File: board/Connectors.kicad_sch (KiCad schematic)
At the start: 17 parts, among them J10 SLOT 1, J11 SLOT 2, J12 SLOT 3, J13 SLOT 4, J14 SLOT 5, J15 Audio Jack, J16 SPI Device 0, J18 SPI Device 1, J19 SPI Device 2, J20 SPI Device 3, J21 SPI Device 4, J22 SPI Device 5, J23 SPI Device 6, J24 SPI Device 7, J25 VIA Port A, J26 SP720APP, J9 SLOT 0

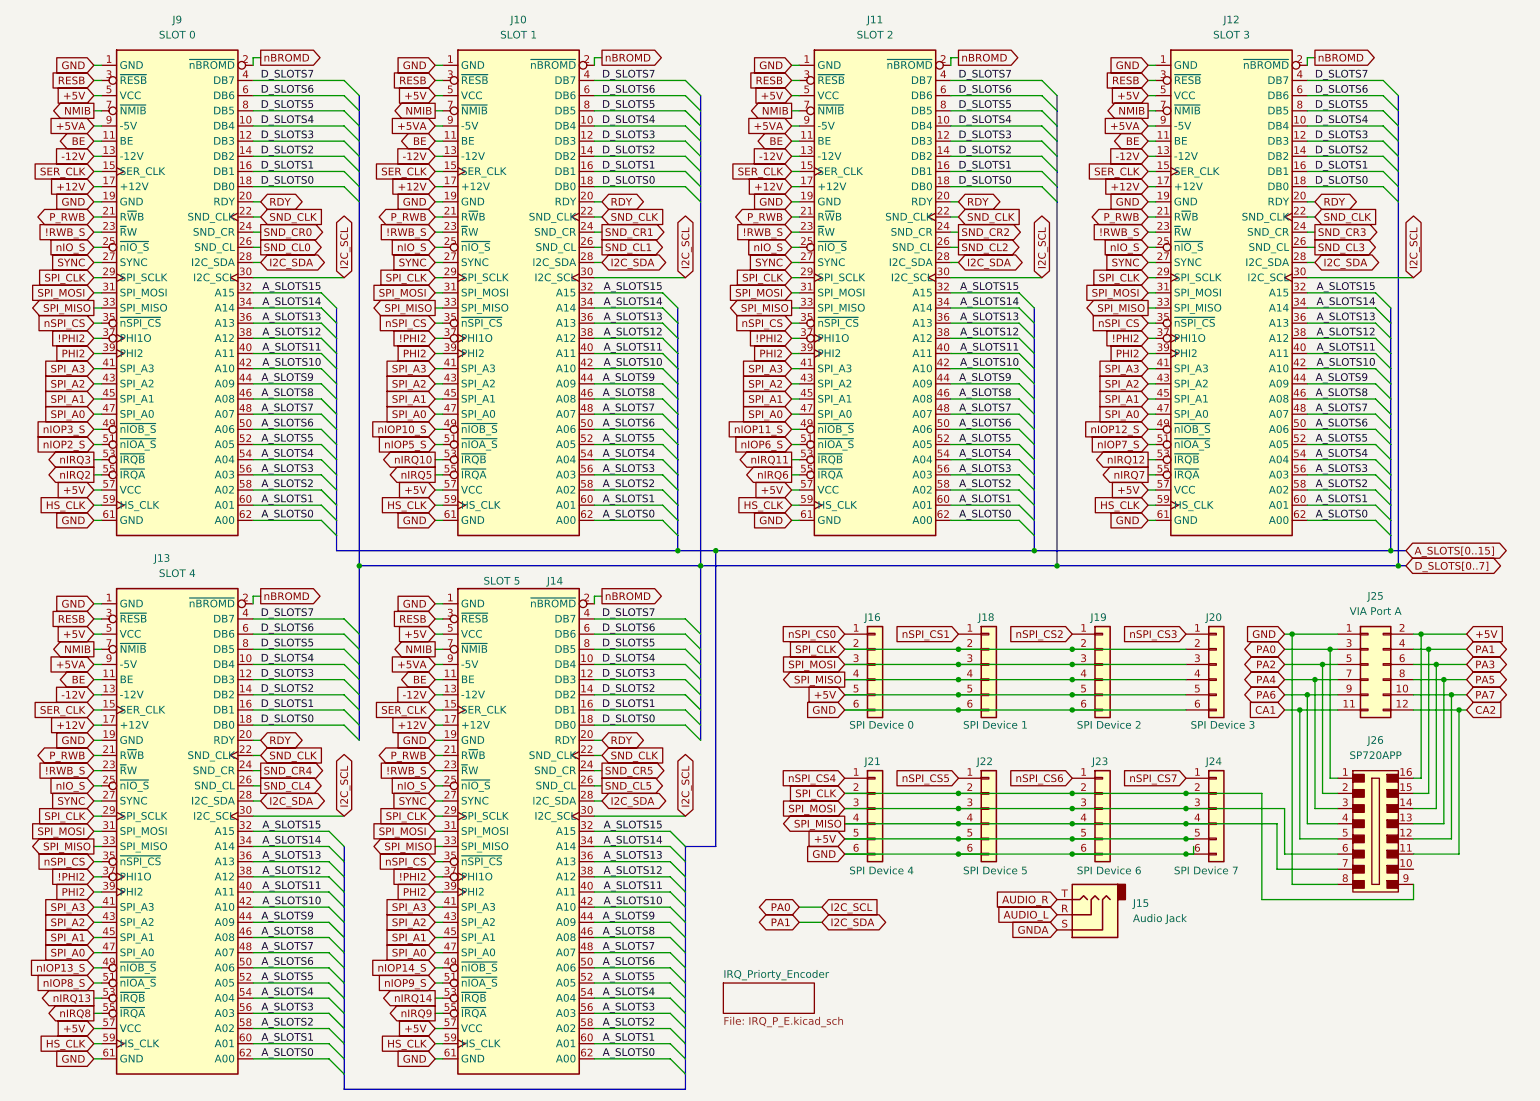
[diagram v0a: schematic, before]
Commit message: V1.4E
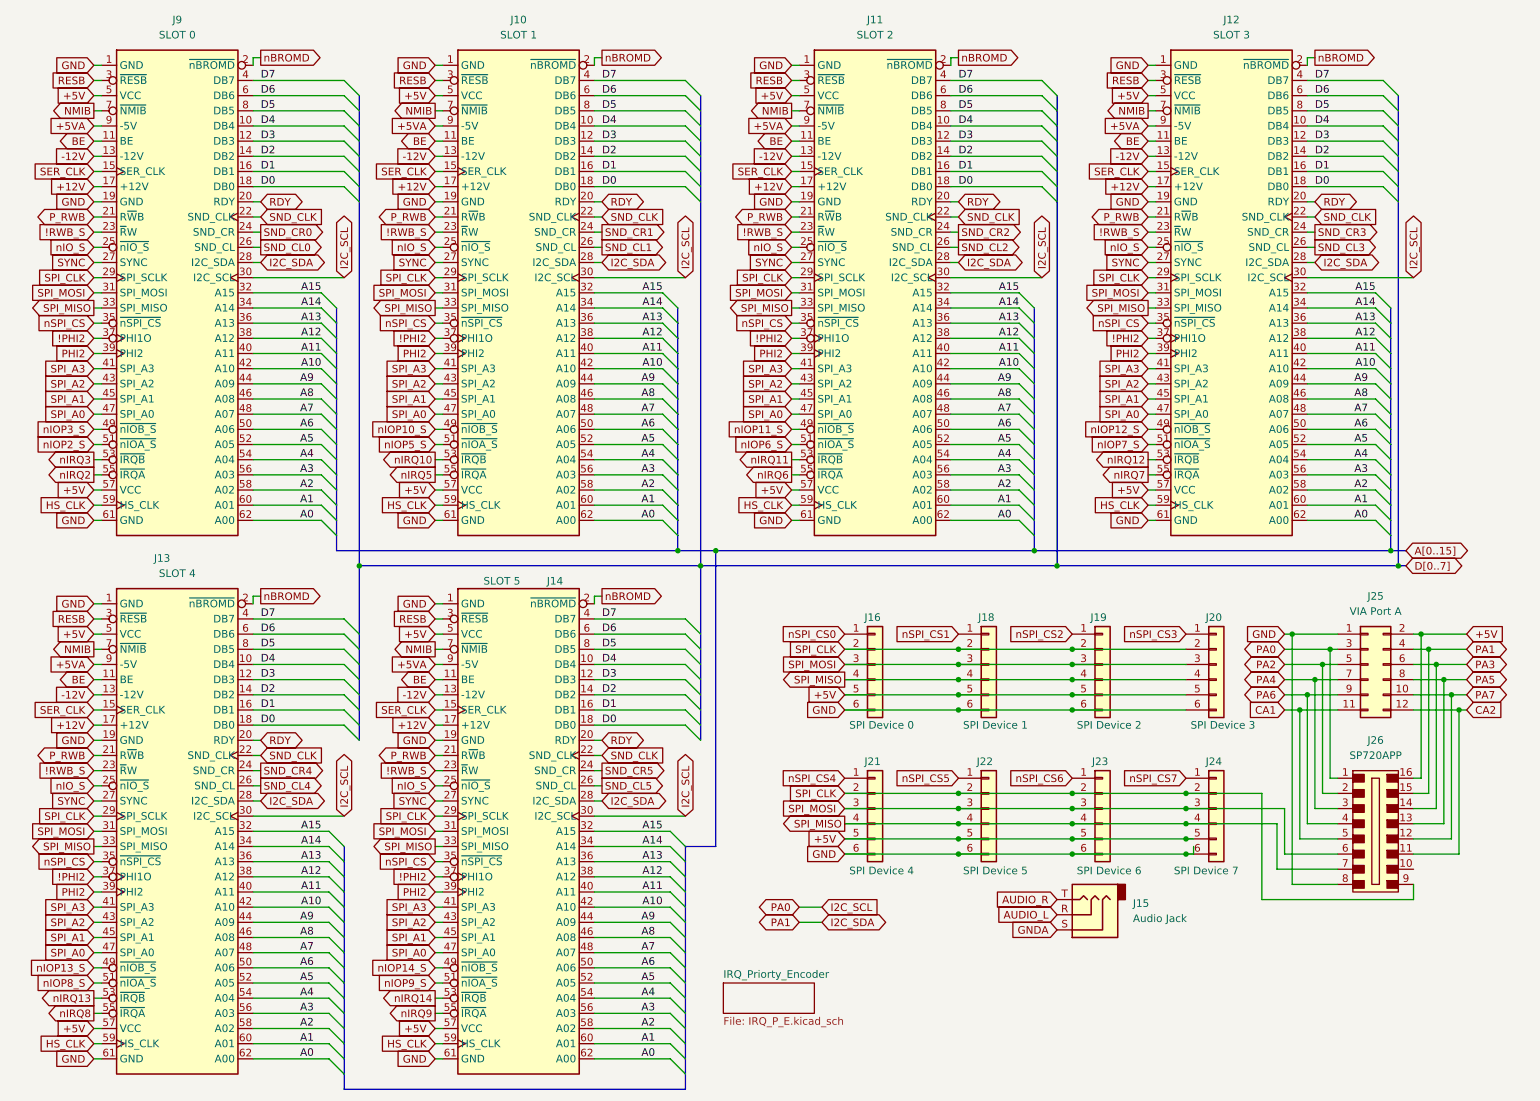
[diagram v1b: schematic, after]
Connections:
- net A_SLOTS0 renamed A0
- net A_SLOTS1 renamed A1
- net A_SLOTS10 renamed A10
- net A_SLOTS11 renamed A11
- net A_SLOTS12 renamed A12
- net A_SLOTS13 renamed A13
- net A_SLOTS14 renamed A14
- net A_SLOTS15 renamed A15
- net A_SLOTS2 renamed A2
- net A_SLOTS3 renamed A3
- net A_SLOTS4 renamed A4
- net A_SLOTS5 renamed A5
- net A_SLOTS6 renamed A6
- net A_SLOTS7 renamed A7
- net A_SLOTS8 renamed A8
- net A_SLOTS9 renamed A9
- net D_SLOTS0 renamed D0
- net D_SLOTS1 renamed D1
- net D_SLOTS2 renamed D2
- net D_SLOTS3 renamed D3
- net D_SLOTS4 renamed D4
- net D_SLOTS5 renamed D5
- net D_SLOTS6 renamed D6
- net D_SLOTS7 renamed D7
